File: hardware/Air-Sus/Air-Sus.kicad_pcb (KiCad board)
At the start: 2 copper layers, 54 x 65.4 mm, 43 parts, among them IC1 ABPMRRV060MG2A3, IC2 ABPMRRV060MG2A3, J1 53307-2471, J2 Conn_01x05, J5 MX150_02x08_Vertical, U1 Opamp_Dual, U2 LDO40LPURY

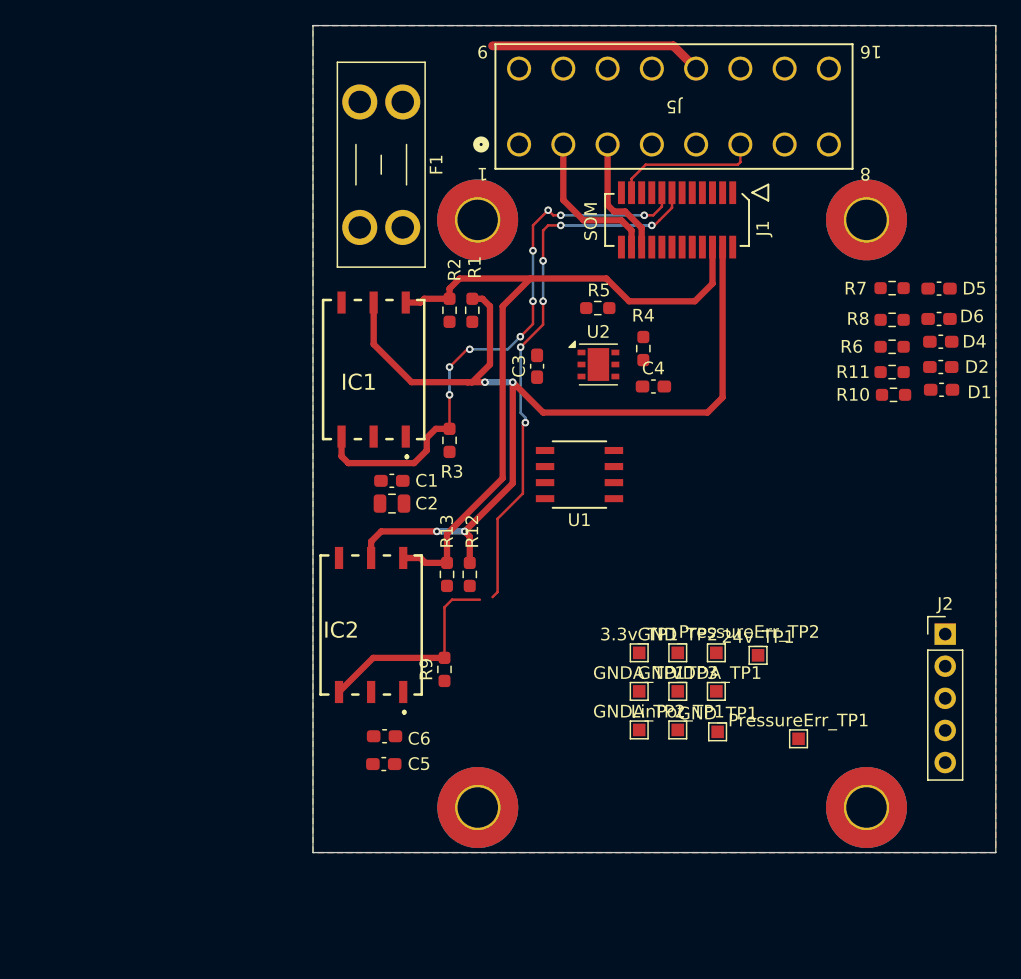
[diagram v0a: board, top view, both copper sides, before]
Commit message: air-sus layout check e Please enter the commit message for your changes. Lines starting
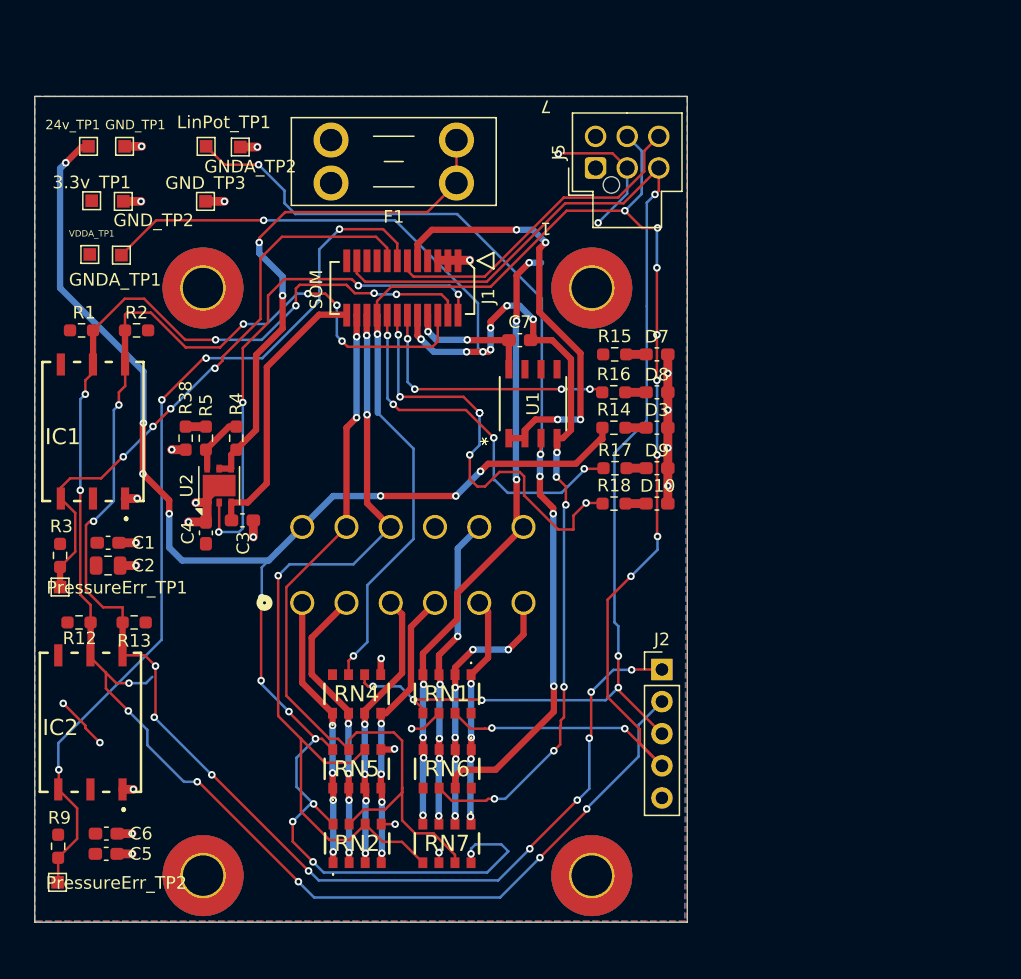
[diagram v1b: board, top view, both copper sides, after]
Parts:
- removed D1, D2, D4, D5, D6: LED, Capacitor_SMD:C_0603_1608Metric_Pad1.08x0.95mm_HandSolder
- removed R10, R11, R6, R7, R8: 100, Resistor_SMD:R_0603_1608Metric_Pad0.98x0.95mm_HandSolder
- added C7: 0.1uF, Capacitor_SMD:C_0603_1608Metric_Pad1.08x0.95mm_HandSolder, F.Cu at (125.4, 48.5)
- added D10: LED, Capacitor_SMD:C_0603_1608Metric_Pad1.08x0.95mm_HandSolder, F.Cu at (136.2, 61.4)
- added D3: LED, Capacitor_SMD:C_0603_1608Metric_Pad1.08x0.95mm_HandSolder, F.Cu at (136.2, 55.4)
- added D7: LED, Capacitor_SMD:C_0603_1608Metric_Pad1.08x0.95mm_HandSolder, F.Cu at (136.2, 49.6)
- added D8: LED, Capacitor_SMD:C_0603_1608Metric_Pad1.08x0.95mm_HandSolder, F.Cu at (136.2, 52.6)
- added D9: LED, Capacitor_SMD:C_0603_1608Metric_Pad1.08x0.95mm_HandSolder, F.Cu at (136.2, 58.6)
- added J4: MX150_02x06_Vertical, UTSVT_Connectors:MX150_02x06_Vertical, B.Cu at (108.1, 69.2)
- added R14: 1k, Resistor_SMD:R_0603_1608Metric_Pad0.98x0.95mm_HandSolder, F.Cu at (132.8, 55.4)
- added R15: 1k, Resistor_SMD:R_0603_1608Metric_Pad0.98x0.95mm_HandSolder, F.Cu at (132.9, 49.6)
- added R16: 1k, Resistor_SMD:R_0603_1608Metric_Pad0.98x0.95mm_HandSolder, F.Cu at (132.8, 52.6)
- added R17: 1k, Resistor_SMD:R_0603_1608Metric_Pad0.98x0.95mm_HandSolder, F.Cu at (132.9, 58.6)
- added R18: 1k, Resistor_SMD:R_0603_1608Metric_Pad0.98x0.95mm_HandSolder, F.Cu at (132.8, 61.4)
- added R38: 2.49k, Resistor_SMD:R_0603_1608Metric_Pad0.98x0.95mm_HandSolder, F.Cu at (98.9, 56.2)
- added RN1: YC324-JK-070RL, 4pinRes:YC324JK07220RL, F.Cu at (119.6, 76.5)
- added RN2: YC324-JK-070RL, 4pinRes:YC324JK07220RL, F.Cu at (112.5, 88.3)
- added RN4: YC324-JK-070RL, 4pinRes:YC324JK07220RL, F.Cu at (112.5, 76.5)
- added RN5: YC324-JK-070RL, 4pinRes:YC324JK07220RL, F.Cu at (112.5, 82.4)
- added RN6: YC324-JK-070RL, 4pinRes:YC324JK07220RL, F.Cu at (119.6, 82.4)
- added RN7: YC324-JK-070RL, 4pinRes:YC324JK07220RL, F.Cu at (119.6, 88.3)
- J5: value MX150_02x08_Vertical -> Conn_01x06; footprint UTSVT_Connectors:CONN16_0757575481_MOL -> Connector_Molex:Molex_Nano-Fit_105310-xx06_2x03_P2.50mm_Vertical
- R5: value 17.5k -> 15k
- moved 24v_TP1 66.5 mm to (91.2, 33.1)
- moved GND_TP1 65.9 mm to (94.1, 33.1)
- moved VDDA_TP1 60.4 mm to (91.3, 41.7)
- moved PressureErr_TP1 59.6 mm to (89.0, 68.0)
- moved LinPot_TP1 59.3 mm to (100.5, 33.1)
- moved GND_TP2 56.5 mm to (94.0, 37.5)
- moved 3.3v_TP1 56.2 mm to (91.5, 37.5)
- moved GNDA_TP2 55.9 mm to (103.2, 33.2)
- moved PressureErr_TP2 55.2 mm to (88.8, 91.3)
- moved GND_TP3 53.8 mm to (100.5, 37.5)
- moved GNDA_TP1 53.5 mm to (93.8, 41.8)
- moved C4 37.2 mm to (100.5, 63.7), turned to 90 degrees
- moved R9 33.6 mm to (88.8, 88.5), turned to -90 degrees
- moved R4 33.0 mm to (102.9, 56.2)
- moved R5 32.7 mm to (100.5, 56.2), turned to 90 degrees
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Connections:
- net /SCL2 renamed SCL2
- J1 pad 12: /diff_status -> diff_status
- J1 pad 14: /Temp_status -> Temp_status
- J1 pad 16: /ir_status -> ir_status
- J1 pad 20: /CAN_L -> CAN_L
- J1 pad 21: /SDA2 -> SDA2
- J1 pad 22: /CAN_H -> CAN_H
- J1 pad 9: /linpot12_out -> /linpot_norm
- J2 pad 3: /SDA2 -> SDA2
- J5 pad 1: +24V -> unconnected-(J5-Pin_1-Pad1)
- J5 pad 2: /CAN_H -> GND
- J5 pad 3: /CAN_L -> SDA2
- J5 pad 4: +24V -> +3.3V
- J5 pad 6: /SDA2 -> /IR_STAT
- LinPot_TP1 pad 1: /linpot12_out -> linpot_out
- R5 pad 2: GND -> Net-(R38-Pad1)
- U1 pad 3: /linpot_out -> linpot_out
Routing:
- net +24V: track 0.00 -> 130.5 mm, vias 0 -> 15
- net SCL2: track 0.00 -> 129.6 mm, vias 0 -> 12
- net GNDA: track 0.00 -> 99.8 mm, vias 0 -> 14
- net SDA2: track 0.00 -> 99.7 mm, vias 0 -> 6
- net linpot_out: track 0.00 -> 77.5 mm, vias 0 -> 5
- net /SCL: track 58.6 -> 127.6 mm, vias 0 -> 15
- net CAN_L: track 0.00 -> 66.2 mm, vias 0 -> 3
- net CAN_H: track 0.00 -> 62.5 mm, vias 0 -> 2
- net GND: track 0.00 -> 57.8 mm, vias 0 -> 28
- net /mx150Connector/Gen_8: track 0.00 -> 49.4 mm, vias 0 -> 7
- net /SDA: track 79.2 -> 128.0 mm, vias 4 -> 12
- net Net-(U2-Vout): track 0.00 -> 42.4 mm, vias 0 -> 2
- net /3.3MCU: track 0.00 -> 41.3 mm, vias 0 -> 4
- net Temp_status: track 0.00 -> 34.8 mm, vias 0 -> 6
- net /linpot_norm: track 0.00 -> 34.5 mm, vias 0 -> 4
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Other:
- board size 54 x 65.4 mm -> 51.6 x 65.3 mm
- board text added: "*"
- board text added: "1 7"

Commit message: finished rev a layout for all 3 boards + added cubemx file
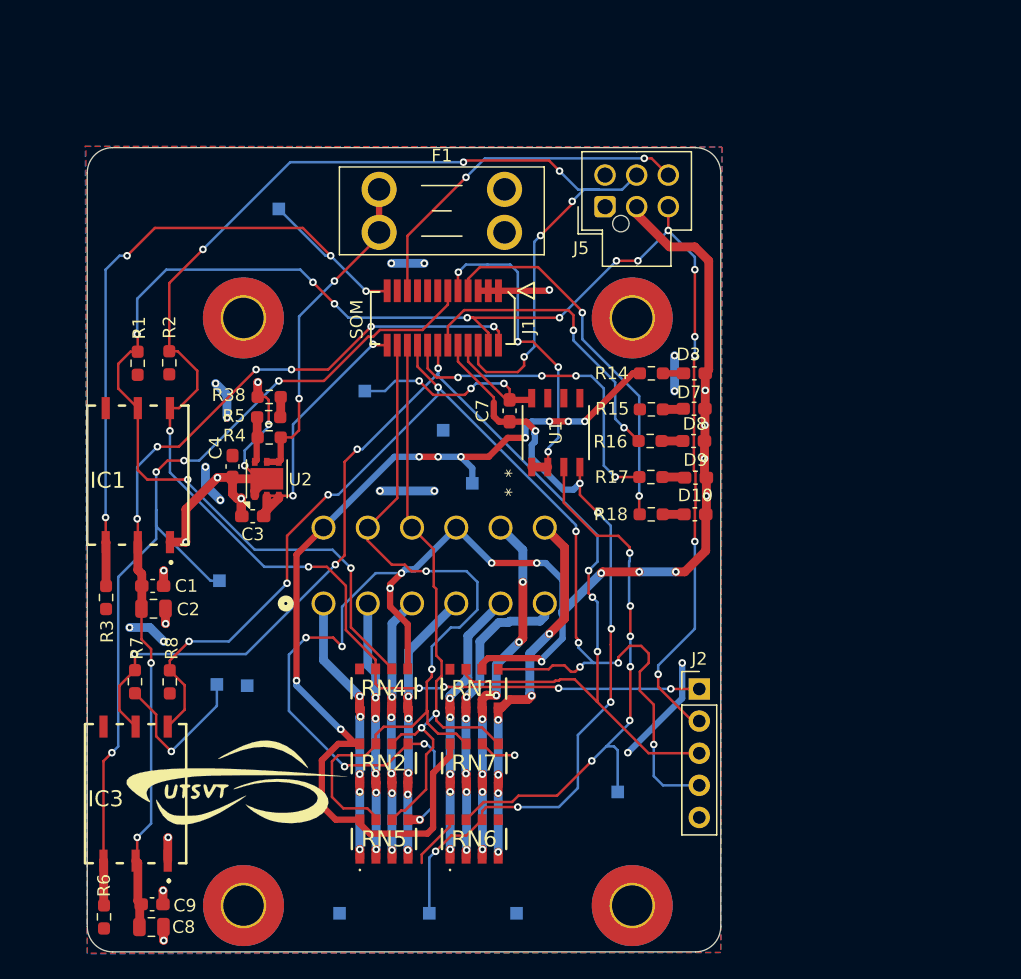
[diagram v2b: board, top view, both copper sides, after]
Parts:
- removed C5: 10uf, Capacitor_SMD:C_0603_1608Metric_Pad1.08x0.95mm_HandSolder
- removed C6: 0.1uF, Capacitor_SMD:C_0603_1608Metric_Pad1.08x0.95mm_HandSolder
- removed IC2: ABPMRRV060MG2A3, footprints:ABPMRRV060MG2A3
- removed R12, R13, R9: 4.7k, Resistor_SMD:R_0603_1608Metric_Pad0.98x0.95mm_HandSolder
- added C8: 10uf, Capacitor_SMD:C_0805_2012Metric, F.Cu at (96.2, 94.9)
- added C9: 0.1uF, Capacitor_SMD:C_0603_1608Metric_Pad1.08x0.95mm_HandSolder, F.Cu at (96.3, 93.1)
- added G***: LOGO, UTSVT_Logos:UTSVT_Logo_Symbol, F.Cu at (102.7, 83.6)
- added G***: LHRs_LOGO, UTSVT_Logos:LHRs_LOGO, F.Cu at (100.6, 37.5)
- added IC3: ABPMRRV060MG2A3, footprints:ABPMRRV060MG2A3, F.Cu at (95.0, 84.3)
- added R6: 4.7k, Resistor_SMD:R_0603_1608Metric_Pad0.98x0.95mm_HandSolder, F.Cu at (92.5, 94.1)
- added R7: 4.7k, Resistor_SMD:R_0603_1608Metric_Pad0.98x0.95mm_HandSolder, F.Cu at (94.9, 75.5)
- added R8: 4.7k, Resistor_SMD:R_0603_1608Metric_Pad0.98x0.95mm_HandSolder, F.Cu at (97.7, 75.5)
- 24v_TP1, 3.3v_TP1, GNDA_TP1, GNDA_TP2, GND_TP1, GND_TP2, GND_TP3, LinPot_TP1, PressureErr_TP1, PressureErr_TP2, VDDA_TP1: moved to B.Cu
- moved GND_TP3 61.4 mm to (125.1, 93.8), turned to 180 degrees
- moved GNDA_TP2 61.1 mm to (111.1, 93.8), turned to 180 degrees
- moved LinPot_TP1 60.5 mm to (133.1, 84.2), turned to 180 degrees
- moved GNDA_TP1 57.5 mm to (118.2, 93.8), turned to 180 degrees
- moved 24v_TP1 40.4 mm to (121.6, 59.8)
- moved GND_TP2 39.5 mm to (103.8, 75.8), turned to 180 degrees
- moved 3.3v_TP1 39.5 mm to (101.4, 75.7), turned to 180 degrees
- moved PressureErr_TP1 34.5 mm to (106.3, 38.1), turned to 180 degrees
- moved GND_TP1 33.7 mm to (119.3, 55.6), turned to 180 degrees
- moved PressureErr_TP2 27.1 mm to (101.6, 67.5), turned to 180 degrees
- moved VDDA_TP1 24.3 mm to (113.1, 52.5), turned to 180 degrees
- moved R38 7.36 mm to (105.5, 53.0), turned to 180 degrees
- moved RN7 6.71 mm to (121.8, 81.9), turned to 0 degrees
- moved RN2 6.69 mm to (114.6, 81.9)
- moved F1 6.14 mm to (114.2, 36.5), turned to 0 degrees
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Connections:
- net CAN_H renamed /CAN_H
- net CAN_L renamed /CAN_L
- net diff_status renamed /diff_status
- net ir_status renamed /ir_status
- C1 pad 1: +3.3V -> +3.3V MCU
- C2 pad 1: +3.3V -> +3.3V MCU
- IC1 pad 2: +3.3V -> +3.3V MCU
- J1 pad 11: /IR_STAT -> /pressure_err2
- J1 pad 13: /pressure_err2 -> unconnected-(J1-ADC1_IN10-Pad13)
- J1 pad 14: Temp_status -> /SDA2
- J1 pad 15: /pressure_err1 -> unconnected-(J1-ADC1_IN11-Pad15)
- J1 pad 18: SCL2 -> /SCL2
- J1 pad 19: unconnected-(J1-SPI1_NSS-Pad19) -> /IR_INTER
- J1 pad 2: /3.3MCU -> +3.3V MCU
- J1 pad 21: SDA2 -> unconnected-(J1-SPI1_MISO-Pad21)
- J1 pad 23: unconnected-(J1-SPI1_SCK-Pad23) -> /pressure_err1
- J1 pad 7: unconnected-(J1-OPAMP1_VINP-Pad7) -> /Temp_status
- J2 pad 3: SDA2 -> /SDA2
- J2 pad 4: SCL2 -> /SCL2
- J5 pad 3: SDA2 -> /SDA
- J5 pad 5: SCL2 -> /SCL
- J5 pad 6: /IR_STAT -> /IR_INTER
- R18 pad 1: Temp_status -> /Temp_status
- RN1 pad 5: SDA2 -> /SCL2
- RN1 pad 7: SCL2 -> /SDA2
- RN4 pad 6: SDA2 -> /SDA
- RN4 pad 7: SCL2 -> /SCL
- U2 pad 2: /3.3MCU -> /24v_out
- VDDA_TP1 pad 1: +VDDA -> VDDA
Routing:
- net SCL2: track 129.6 -> 0.00 mm, vias 12 -> 0
- net GND: track 57.8 -> 164.6 mm, vias 28 -> 30
- net /SDA2: track 0.00 -> 100.4 mm, vias 0 -> 7
- net SDA2: track 99.7 -> 0.00 mm, vias 6 -> 0
- net /SCL2: track 0.00 -> 97.8 mm, vias 0 -> 9
- net +3.3V MCU: track 0.00 -> 72.1 mm, vias 0 -> 8
- net +24V: track 130.5 -> 77.7 mm, vias 15 -> 9
- net +3.3V: track 0.01 -> 45.4 mm, vias 0 -> 15
- net /3.3MCU: track 41.3 -> 0.00 mm, vias 4 -> 0
- net GNDA: track 99.8 -> 64.5 mm, vias 14 -> 7
- net Temp_status: track 34.8 -> 0.00 mm, vias 6 -> 0
- net linpot_out: track 77.5 -> 44.0 mm, vias 5 -> 6
- net /Temp_status: track 0.00 -> 29.7 mm, vias 0 -> 2
- net /IR_INTER: track 0.00 -> 28.1 mm, vias 0 -> 2
- net /IR_STAT: track 27.1 -> 0.00 mm
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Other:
- board size 51.6 x 65.3 mm -> 50.1 x 63.6 mm
- board text removed: "*"
- board text removed: "1 7"
